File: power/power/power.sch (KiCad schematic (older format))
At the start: 41 parts, among them J1 BEXUS 28V, U1 INA181, U2 INA181, U3 INA181

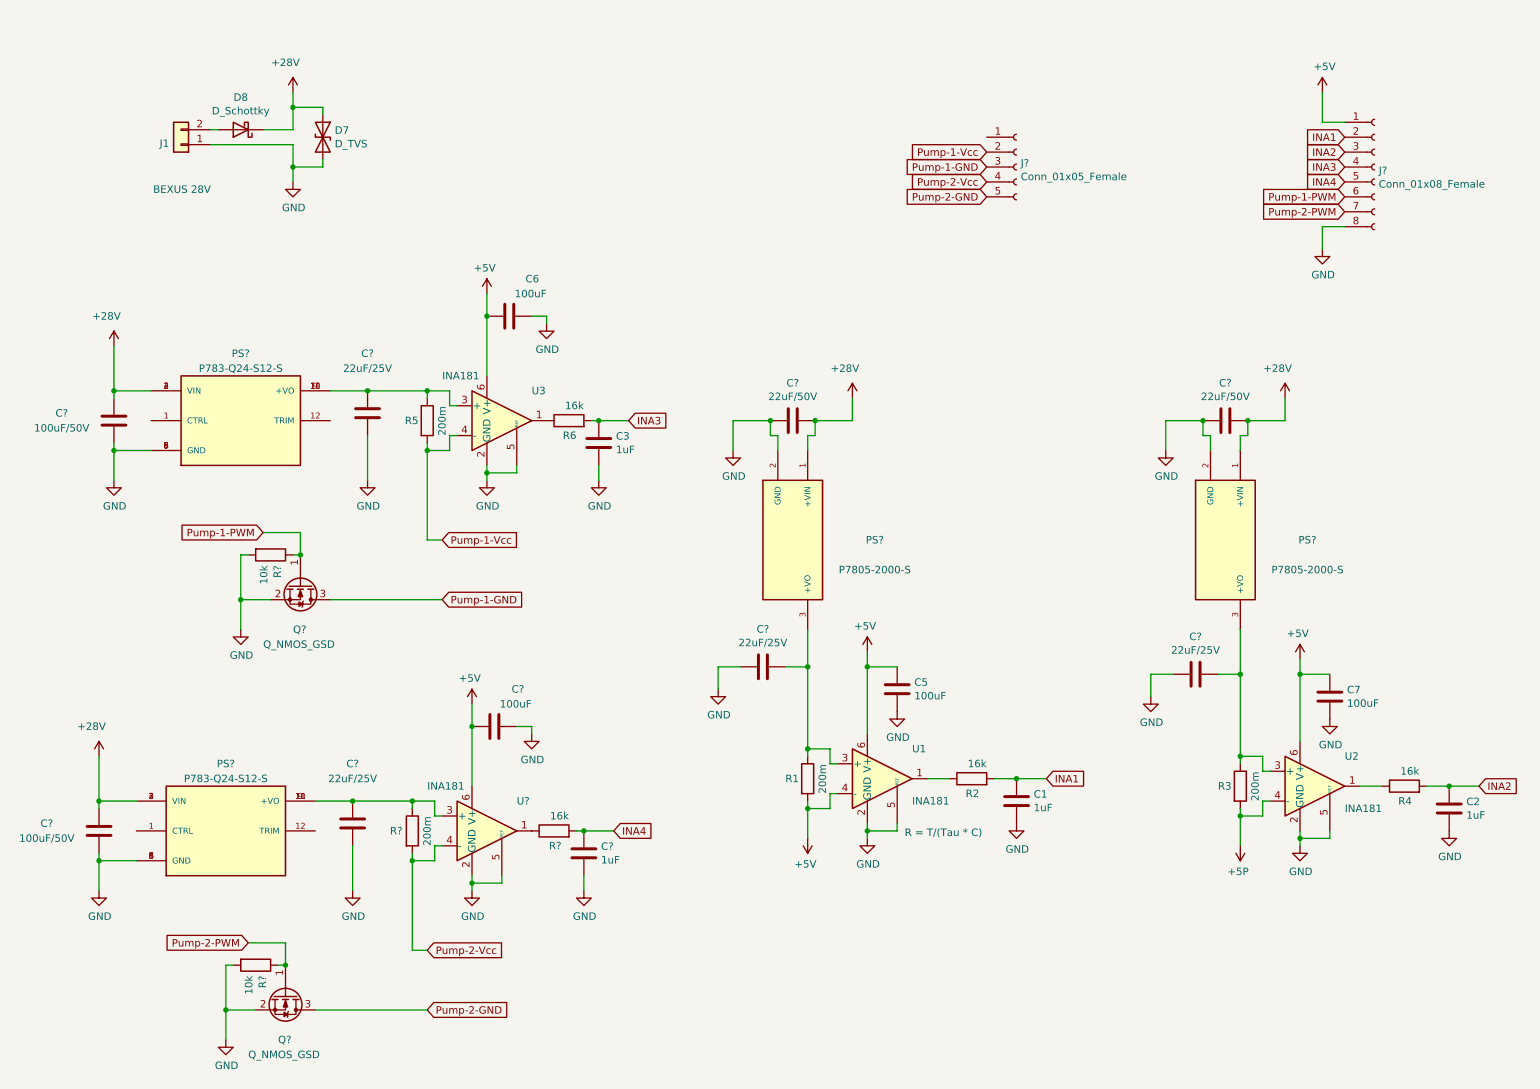
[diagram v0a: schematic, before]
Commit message: change everything
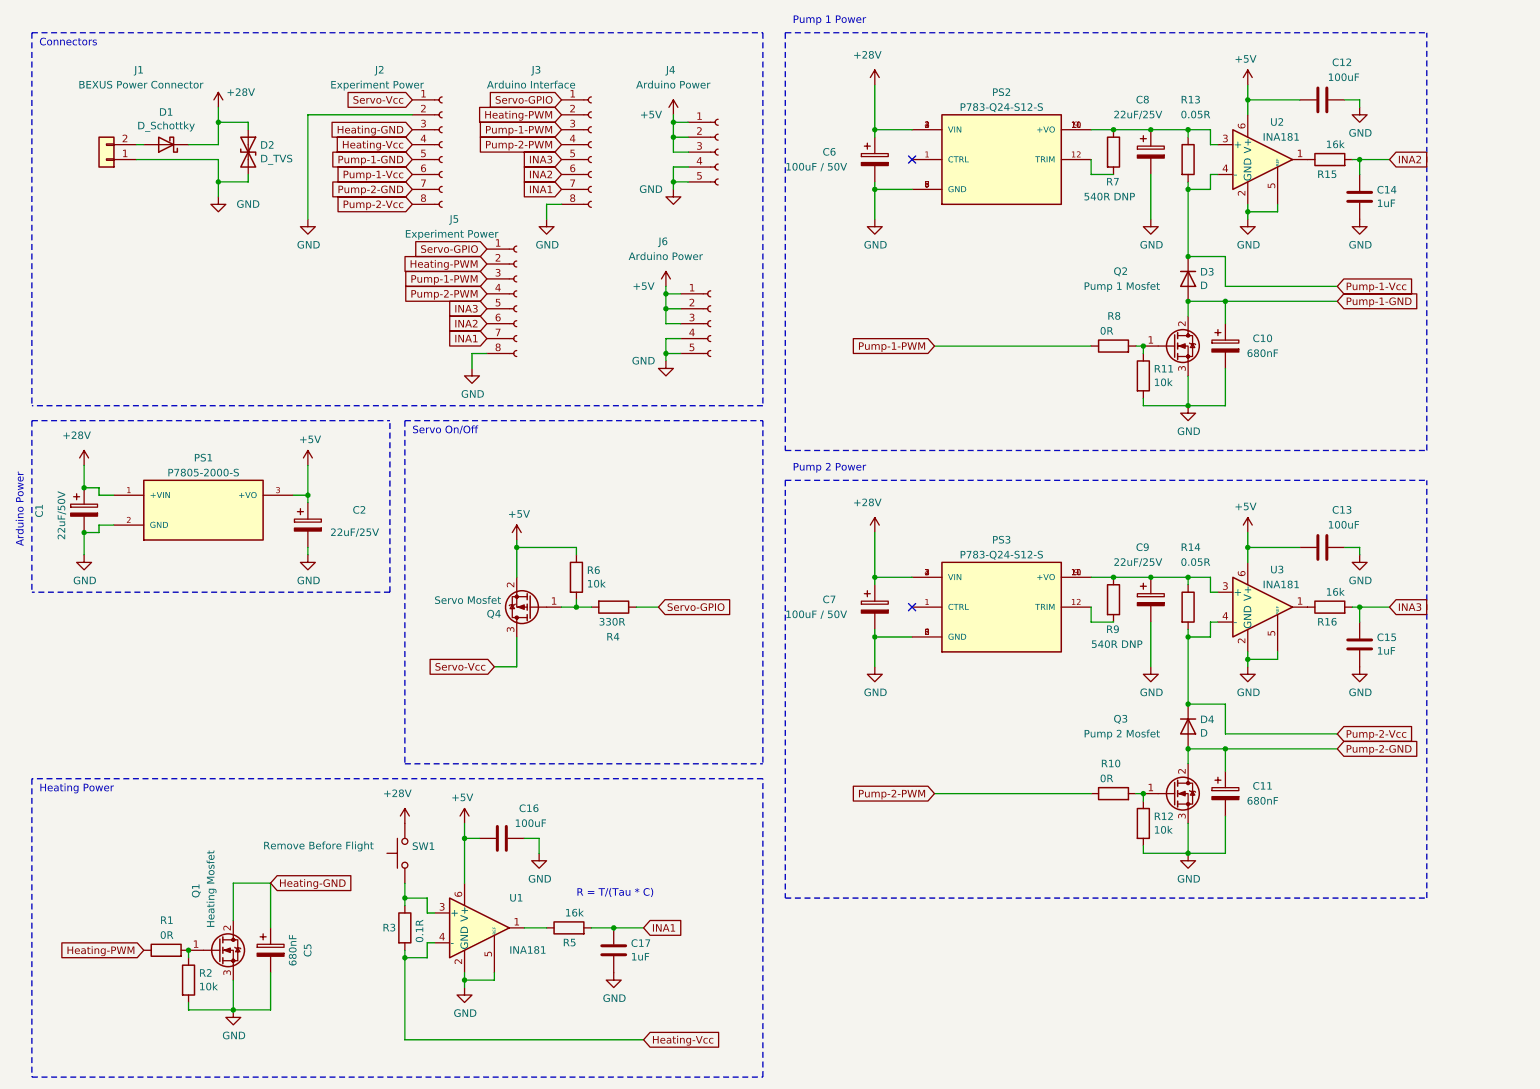
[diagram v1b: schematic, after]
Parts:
- removed C1, C2, C3, C?: 1uF, Capacitor_SMD:C_0603_1608Metric_Pad1.05x0.95mm_HandSolder, symbol Device:C
- removed C5, C6, C7, C?: 100uF, Capacitor_SMD:C_0603_1608Metric_Pad1.05x0.95mm_HandSolder, symbol Device:C
- removed C? (x2): 22uF/50V, symbol Device:C
- removed C? (x2): 100uF/50V, symbol Device:C
- removed C? (x4): 22uF/25V, symbol Device:C
- removed J?: Conn_01x05_Female, symbol Connector:Conn_01x05_Female
- removed PS?: P7805-2000-S, CONV_P7805-2000-S, symbol Stardust:P7805-2000-S
- removed PS? (x2): P783-Q24-S12-S, CONV_P783-Q24-S12-S, symbol Stardust:P783-Q24-S12-S
- removed Q? (x2): Q_NMOS_GSD, symbol Device:Q_NMOS_GSD
- removed R?: 200m, Resistor_SMD:R_0603_1608Metric_Pad1.05x0.95mm_HandSolder, symbol Device:R
- removed R?: 16k, Resistor_SMD:R_0603_1608Metric_Pad1.05x0.95mm_HandSolder, symbol Device:R
- removed R? (x2): 10k, symbol Device:R
- removed U?: INA181, Package_TO_SOT_SMD:SOT-23-6, symbol Amplifier_Current:INA181
- added C1: 22uF/50V, Capacitor_THT:CP_Radial_D5.0mm_P2.50mm, symbol Device:CP
- added C10, C11, C5: 680nF, Capacitor_THT:CP_Radial_D5.0mm_P2.50mm, symbol Device:CP
- added C12, C13, C16: 100uF, Capacitor_SMD:C_0603_1608Metric_Pad1.08x0.95mm_HandSolder, symbol Device:C
- added C14, C15, C17: 1uF, Capacitor_SMD:C_0603_1608Metric_Pad1.08x0.95mm_HandSolder, symbol Device:C
- added C2, C8, C9: 22uF/25V, Capacitor_THT:CP_Radial_D5.0mm_P2.50mm, symbol Device:CP
- added C6, C7: 100uF / 50V, Capacitor_THT:CP_Radial_D5.0mm_P2.50mm, symbol Device:CP
- added D3, D4: D, Diode_THT:D_DO-15_P12.70mm_Horizontal, symbol Device:D
- added J2: Experiment Power, Stardust:691382030008, symbol Connector:Conn_01x08_Female
- added J4: Arduino Power, Stardust:691382000005, symbol Connector:Conn_01x05_Female
- added J5: Experiment Power, Connector_PinHeader_2.54mm:PinHeader_1x08_P2.54mm_Vertical, symbol Connector:Conn_01x08_Female
- added J6: Arduino Power, Connector_PinHeader_2.54mm:PinHeader_1x05_P2.54mm_Vertical, symbol Connector:Conn_01x05_Female
- added PS2, PS3: P783-Q24-S12-S, Stardust:CONV_P783-Q24-S12-S, symbol Stardust:P783-Q24-S12-S
- added Q1: Heating Mosfet, Package_TO_SOT_THT:TO-126-3_Horizontal_TabDown, symbol Device:Q_NMOS_GDS
- added Q2: Pump 1 Mosfet, Package_TO_SOT_THT:TO-126-3_Horizontal_TabDown, symbol Device:Q_NMOS_GDS
- added Q3: Pump 2 Mosfet, Package_TO_SOT_THT:TO-126-3_Horizontal_TabDown, symbol Device:Q_NMOS_GDS
- added Q4: Servo Mosfet, Package_TO_SOT_SMD:TSOT-23, symbol Device:Q_PMOS_GSD
- added R10, R8: 0R, Resistor_SMD:R_0603_1608Metric_Pad0.98x0.95mm_HandSolder, symbol Device:R
- added R11, R12: 10k, Resistor_SMD:R_0603_1608Metric_Pad0.98x0.95mm_HandSolder, symbol Device:R
- added R13, R14: 0.05R, Resistor_SMD:R_0603_1608Metric_Pad0.98x0.95mm_HandSolder, symbol Device:R
- added R15, R16: 16k, Resistor_SMD:R_0603_1608Metric_Pad0.98x0.95mm_HandSolder, symbol Device:R
- added R7, R9: 540R DNP, Resistor_SMD:R_0603_1608Metric_Pad0.98x0.95mm_HandSolder, symbol Device:R
- added SW1: Remove Before Flight, Connector_PinHeader_2.54mm:PinHeader_1x02_P2.54mm_Vertical, symbol Switch:SW_Push
- J1: value BEXUS 28V -> BEXUS Power Connector; footprint Connector_Wire:SolderWirePad_1x02_P3.81mm_Drill1.2mm -> Connector_Wire:SolderWire-0.5sqmm_1x02_P4.6mm_D0.9mm_OD2.1mm_Relief
- J3: renamed from J?; value Conn_01x08_Female -> Arduino Interface; footprint (none) -> Stardust:691382030008
- PS1: renamed from PS?; footprint CONV_P7805-2000-S -> Stardust:CONV_P7805-2000-S
- R1: value 200m -> 0R; footprint Resistor_SMD:R_0603_1608Metric_Pad1.05x0.95mm_HandSolder -> Resistor_SMD:R_0603_1608Metric_Pad0.98x0.95mm_HandSolder
- R2, R6: value 16k -> 10k; footprint Resistor_SMD:R_0603_1608Metric_Pad1.05x0.95mm_HandSolder -> Resistor_SMD:R_0603_1608Metric_Pad0.98x0.95mm_HandSolder
- R3: value 200m -> 0.1R; footprint Resistor_SMD:R_0603_1608Metric_Pad1.05x0.95mm_HandSolder -> Resistor_SMD:R_0603_1608Metric_Pad0.98x0.95mm_HandSolder
- R4: value 16k -> 330R; footprint Resistor_SMD:R_0603_1608Metric_Pad1.05x0.95mm_HandSolder -> Resistor_SMD:R_0603_1608Metric_Pad0.98x0.95mm_HandSolder
- R5: value 200m -> 16k; footprint Resistor_SMD:R_0603_1608Metric_Pad1.05x0.95mm_HandSolder -> Resistor_SMD:R_0603_1608Metric_Pad0.98x0.95mm_HandSolder
- renumbered D8 to D1, D7 to D2
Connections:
- net INA4 is gone; now on net INA3: J3.5 (Pin_5)
- net +28V: now also C1.1, C6.1, C7.1, PS2.2 (VIN), PS2.3 (VIN), PS2.4 (VIN), PS3.2 (VIN), PS3.3 (VIN), PS3.4 (VIN), SW1.2
- net +5V: now also PS1.3 (+VO), R6.1, C12.1, C13.1, C16.1, C2.1, J4.1 (Pin_1), J4.2 (Pin_2), J4.3 (Pin_3), J6.1 (Pin_1), J6.2 (Pin_2), J6.3 (Pin_3), Q4.2 (S); no longer J3.1 (Pin_1), R1.2, U1.4 (-)
- net GND: now also R2.2, C1.2, C10.2, C11.2, C12.2, C13.2, C14.2, C15.2, C16.2, C17.2, C2.2, C5.2, C6.2, C7.2, C8.2, C9.2, J2.2 (Pin_2), J4.4 (Pin_4), J4.5 (Pin_5), J5.8 (Pin_8), J6.4 (Pin_4), J6.5 (Pin_5), PS2.5 (GND), PS2.6 (GND), PS2.7 (GND), PS2.8 (GND), PS3.5 (GND), PS3.6 (GND), PS3.7 (GND), PS3.8 (GND), Q1.3 (S), Q2.3 (S), Q3.3 (S), R11.2, R12.2
- net INA1: now also J3.7 (Pin_7), R5.2, C17.1, J5.7 (Pin_7); no longer J3.2 (Pin_2), R2.2
- net INA2: now also J3.6 (Pin_6), C14.1, J5.6 (Pin_6), R15.2; no longer J3.3 (Pin_3), R4.2
- net INA3: now also C15.1, J5.5 (Pin_5), R16.2; no longer J3.4 (Pin_4), R6.2
- net Pump-1-GND: now also C10.1, D3.2 (A), J2.5 (Pin_5), Q2.2 (D)
- net Pump-1-PWM: now also J3.3 (Pin_3), J5.3 (Pin_3), R8.1; no longer J3.6 (Pin_6)
- net Pump-1-Vcc: now also U2.4 (-), D3.1 (K), J2.6 (Pin_6), R13.2; no longer R5.2, U3.4 (-)
- net Pump-2-GND: now also C11.1, D4.2 (A), J2.7 (Pin_7), Q3.2 (D)
- net Pump-2-PWM: now also J3.4 (Pin_4), J5.4 (Pin_4), R10.1; no longer J3.7 (Pin_7)
- net Pump-2-Vcc: now also U3.4 (-), D4.1 (K), J2.8 (Pin_8), R14.2
- net at R2.1: now also R1.2, Q1.1 (G); no longer U1.1
- net at U3.1: now also R16.1; no longer R6.1
- net at U2.1: now also R15.1; no longer R4.1
- net at U2.3 (+): now also C8.1, PS2.10 (+VO), PS2.11 (+VO), PS2.9 (+VO), R13.1, R7.1; no longer R3.1
- net at U3.3 (+): now also C9.1, PS3.10 (+VO), PS3.11 (+VO), PS3.9 (+VO), R14.1, R9.1; no longer R5.1
- net +5P renamed Heating-Vcc
- net Heating-Vcc: now also U1.4 (-), J2.4 (Pin_4); no longer U2.4 (-)
- new net: PS2.12 (TRIM), R7.2
- new net: Q2.1 (G), R11.1, R8.2
- new net: R3.1, SW1.1, U1.3 (+)
- new net: R5.1, U1.1
- new net: Q4.1 (G), R4.2, R6.2
- new net: PS3.12 (TRIM), R9.2
- new net: Q3.1 (G), R10.2, R12.1
- new net Heating-GND: C5.1, J2.3 (Pin_3), Q1.2 (D)
- new net Heating-PWM: J3.2 (Pin_2), J5.2 (Pin_2), R1.1
- new net Servo-GPIO: J3.1 (Pin_1), J5.1 (Pin_1), R4.1
- new net Servo-Vcc: J2.1 (Pin_1), Q4.3 (D)
- no-connect marks 0 -> 2
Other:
- note added: "Arduino Power"
- note added: "Connectors"
- note added: "Heating Power"
- note added: "Pump 1 Power"
- note added: "Pump 2 Power"
- note added: "Servo On/Off"
- moved on the sheet: D1, D2, J1, J3, PS1
